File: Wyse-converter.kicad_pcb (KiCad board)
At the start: 2 copper layers, 39.2 x 53.6 mm, 10 parts, among them J1 4P4C, U1 ProMicro, U2 ProMicro

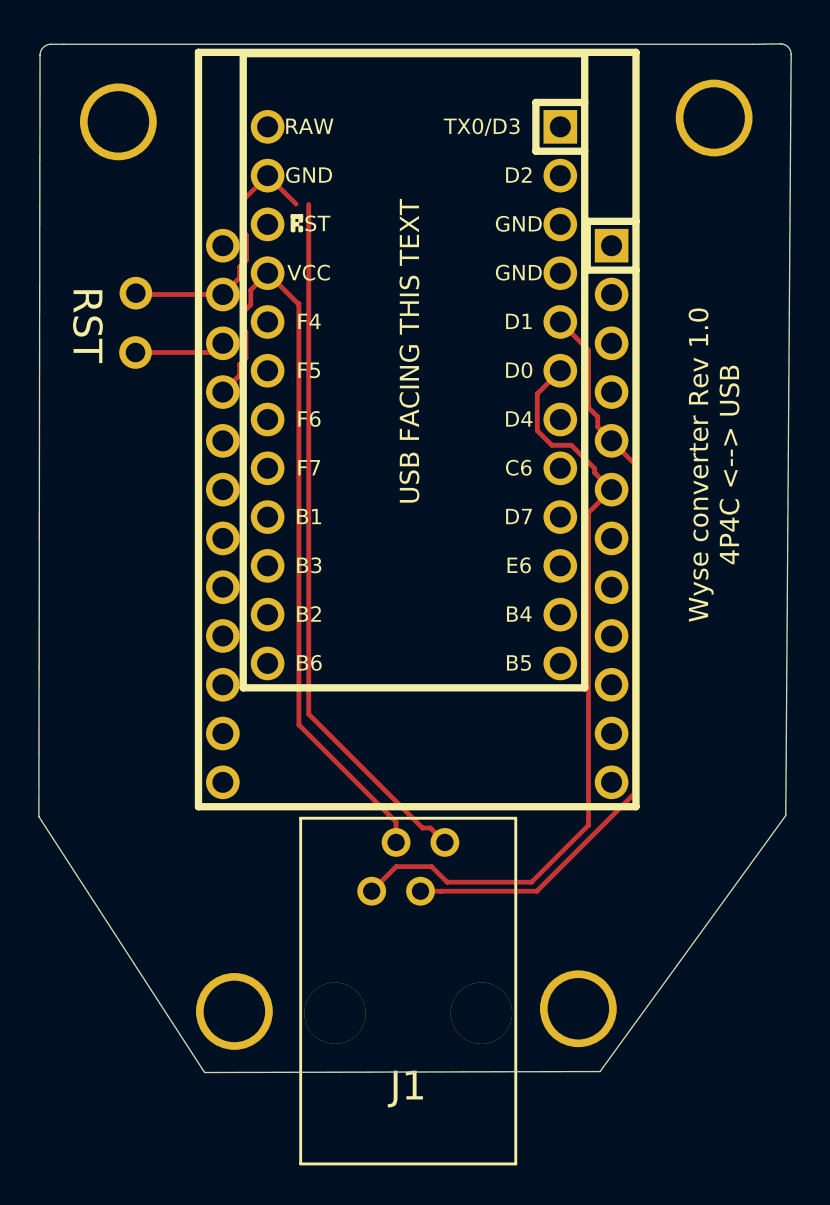
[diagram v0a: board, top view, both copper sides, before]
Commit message: Fixed and working version
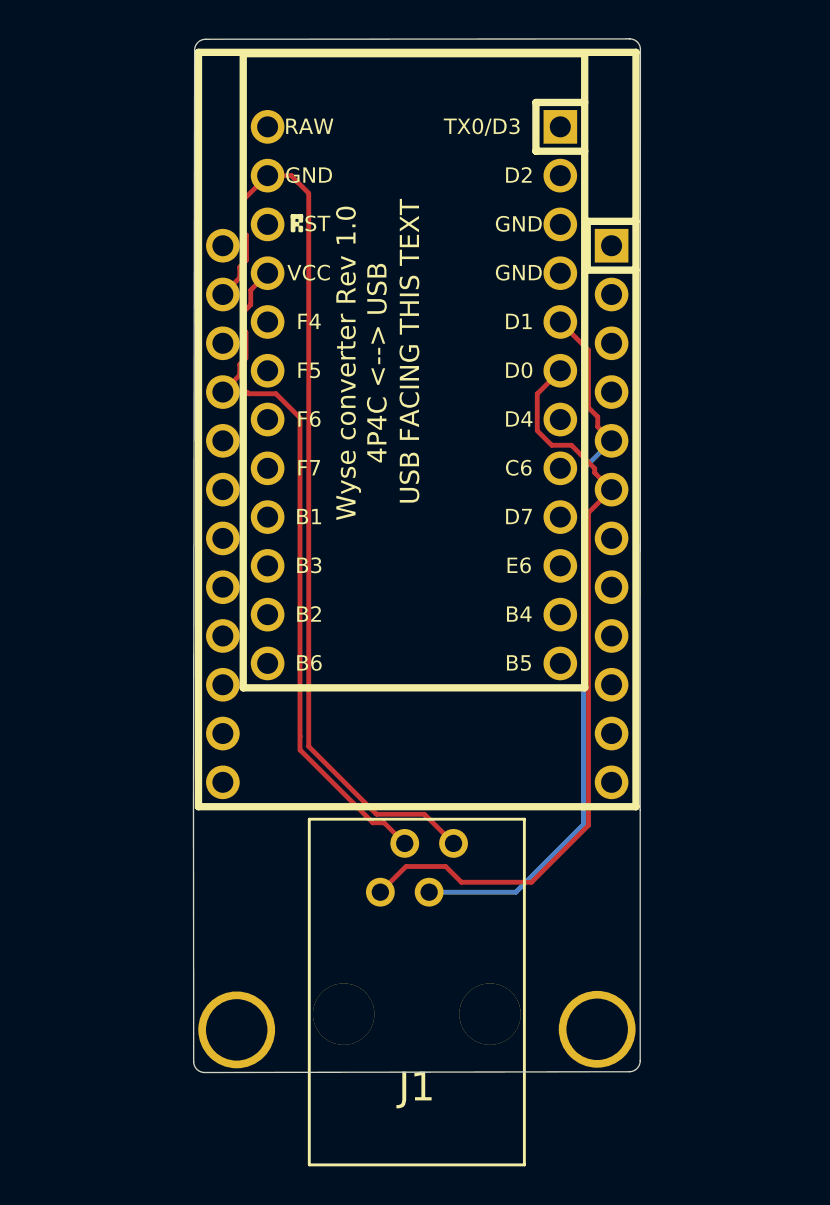
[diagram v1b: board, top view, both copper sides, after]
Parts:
- removed H1, H2: MountingHole, keyboard_parts:HOLE_M3
- removed H5, H6: MountingHole_Pad, keyboard_parts:PIN_1
- moved H4 1.45 mm to (111.9, 99.1)
- moved H3 0.97 mm to (93.1, 99.2)
- moved J1 0.45 mm to (102.5, 98.3)
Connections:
- U1 pad 1: Net-(U1-Pad1) -> (no net)
- U1 pad 10: Net-(U1-Pad10) -> (no net)
- U1 pad 11: Net-(U1-Pad11) -> (no net)
- U1 pad 12: Net-(U1-Pad12) -> (no net)
- U1 pad 13: Net-(U1-Pad13) -> (no net)
- U1 pad 14: Net-(U1-Pad14) -> (no net)
- U1 pad 15: Net-(U1-Pad15) -> (no net)
- U1 pad 16: Net-(U1-Pad16) -> (no net)
- U1 pad 17: Net-(U1-Pad17) -> (no net)
- U1 pad 18: Net-(U1-Pad18) -> (no net)
- U1 pad 19: Net-(U1-Pad19) -> (no net)
- U1 pad 2: Net-(U1-Pad2) -> (no net)
- U1 pad 20: Net-(U1-Pad20) -> (no net)
- U1 pad 22: Net-(U1-Pad22) -> (no net)
- U1 pad 24: Net-(U1-Pad24) -> (no net)
- U1 pad 3: Net-(U1-Pad3) -> (no net)
- U1 pad 4: Net-(U1-Pad4) -> (no net)
- U1 pad 7: Net-(U1-Pad7) -> (no net)
- U1 pad 8: Net-(U1-Pad8) -> (no net)
- U1 pad 9: Net-(U1-Pad9) -> (no net)
- U2 pad 1: Net-(U2-Pad1) -> (no net)
- U2 pad 10: Net-(U2-Pad10) -> (no net)
- U2 pad 11: Net-(U2-Pad11) -> (no net)
- U2 pad 12: Net-(U2-Pad12) -> (no net)
- U2 pad 13: Net-(U2-Pad13) -> (no net)
- U2 pad 14: Net-(U2-Pad14) -> (no net)
- U2 pad 15: Net-(U2-Pad15) -> (no net)
- U2 pad 16: Net-(U2-Pad16) -> (no net)
- U2 pad 17: Net-(U2-Pad17) -> (no net)
- U2 pad 18: Net-(U2-Pad18) -> (no net)
- U2 pad 19: Net-(U2-Pad19) -> (no net)
- U2 pad 2: Net-(U2-Pad2) -> (no net)
- U2 pad 20: Net-(U2-Pad20) -> (no net)
- U2 pad 22: RST -> (no net)
- U2 pad 24: Net-(U2-Pad24) -> (no net)
- U2 pad 3: Net-(U2-Pad3) -> (no net)
- U2 pad 4: Net-(U2-Pad4) -> (no net)
- U2 pad 7: Net-(U2-Pad7) -> (no net)
- U2 pad 8: Net-(U2-Pad8) -> (no net)
- U2 pad 9: Net-(U2-Pad9) -> (no net)
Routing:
- net RST: track 4.75 -> 0.00 mm
- net VCC: track 39.7 -> 36.6 mm
- net GND: track 50.3 -> 48.2 mm
- net CLK: track 39.4 -> 37.4 mm
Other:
- board size 39.2 x 53.6 mm -> 23.3 x 53.8 mm
- board text removed: "RST"
